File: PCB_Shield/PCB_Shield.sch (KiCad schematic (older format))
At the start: 22 parts, among them P1 Power, P2 Analog, P3 Digital, P4 Digital, P5 CONN_01X01, P6 CONN_01X01, P7 CONN_01X01, P8 CONN_01X01, U0 CG, U1 LTC1050, U2 BT_HC-05, U3 Ecran_OLED, U4 Rot_Keyes_KY-040

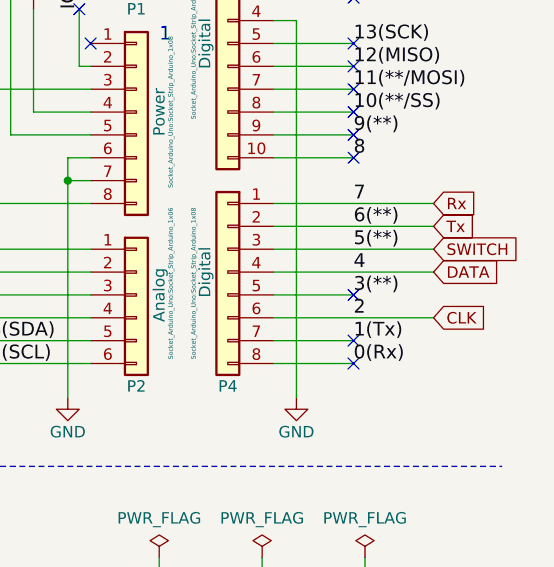
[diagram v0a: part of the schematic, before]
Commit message: Ajout
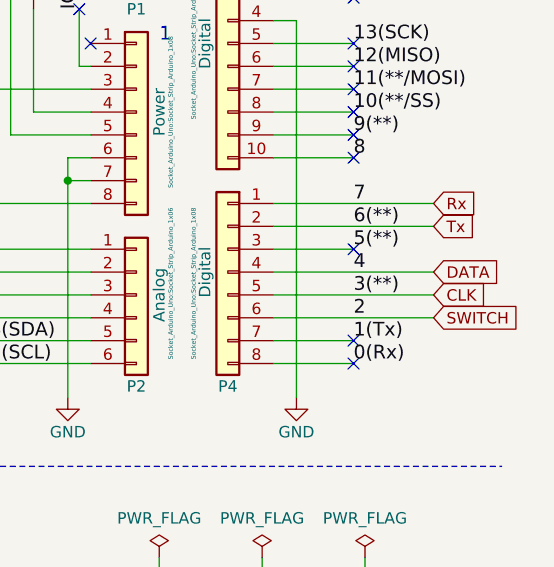
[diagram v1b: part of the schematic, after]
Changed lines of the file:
@@
 Text GLabel 10900 2400 2    50   Input ~ 0
 Tx
-Wire Wire Line
-	10200 2700 10550 2700
-Text GLabel 10900 2800 2    50   Input ~ 0
+Text GLabel 10900 2700 2    50   Input ~ 0
 CLK
 Wire Wire Line
@@
 Wire Wire Line
 	10200 2600 10900 2600
-Text GLabel 10900 2500 2    50   Input ~ 0
+Text GLabel 10900 2800 2    50   Input ~ 0
 SWITCH
-Wire Wire Line
-	10200 2500 10900 2500
 Wire Wire Line
 	10200 2400 10900 2400
@@
 NoConn ~ 10550 2000
 NoConn ~ 10550 2100
-NoConn ~ 10550 2700
 NoConn ~ 10550 3000
 NoConn ~ 4900 2550
@@
 Wire Wire Line
 	2050 2450 1450 2450
+Wire Wire Line
+	10200 2700 10900 2700
+NoConn ~ 10550 2500
+Wire Wire Line
+	10200 2500 10550 2500
 $EndSCHEMATC
